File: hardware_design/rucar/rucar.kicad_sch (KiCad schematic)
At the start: 23 parts

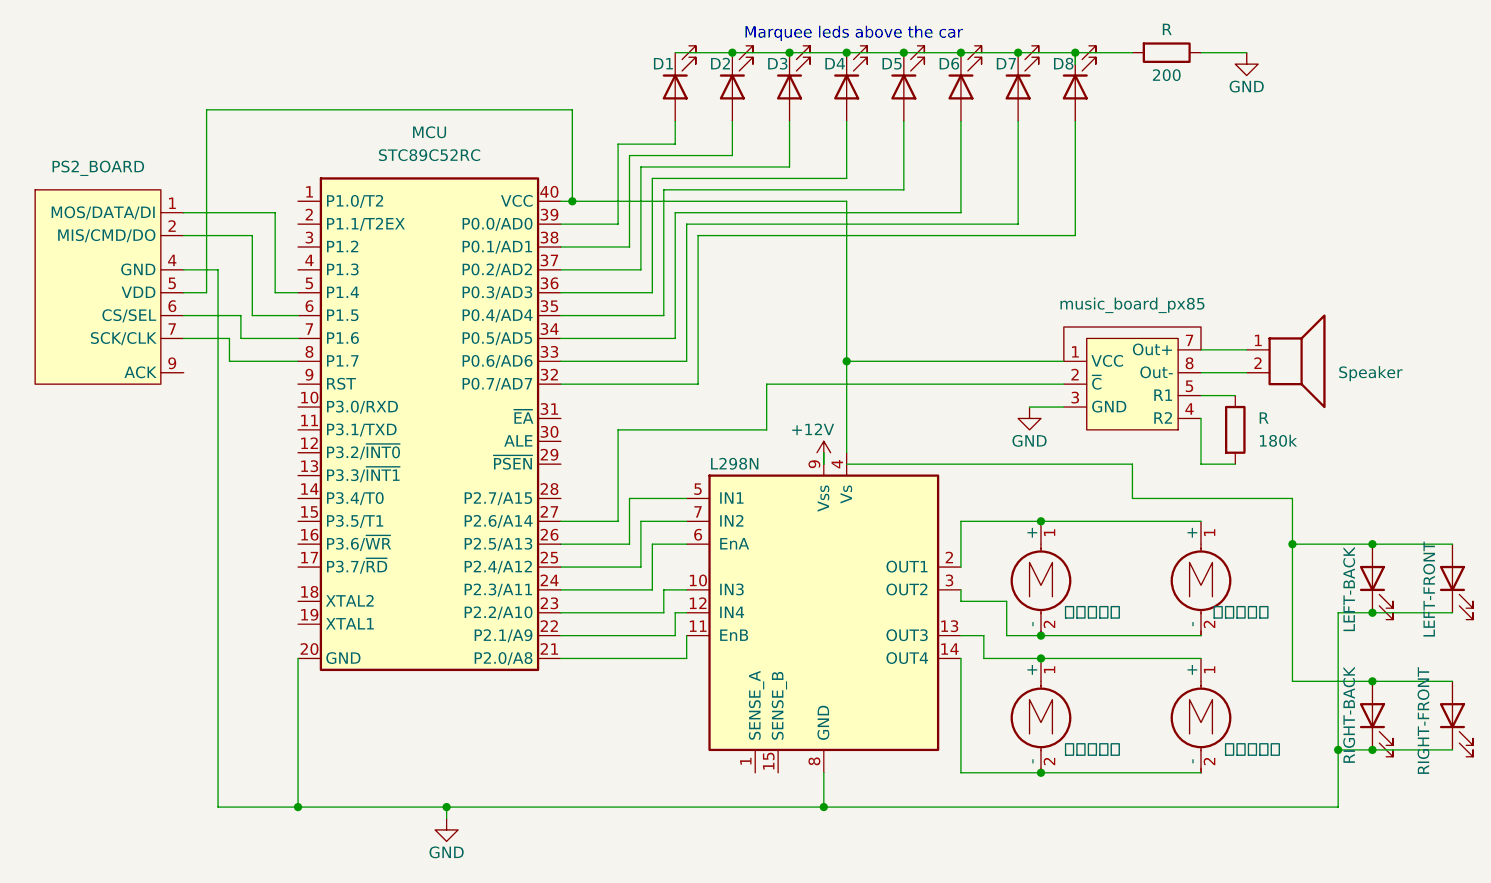
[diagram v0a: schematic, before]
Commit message: optimize
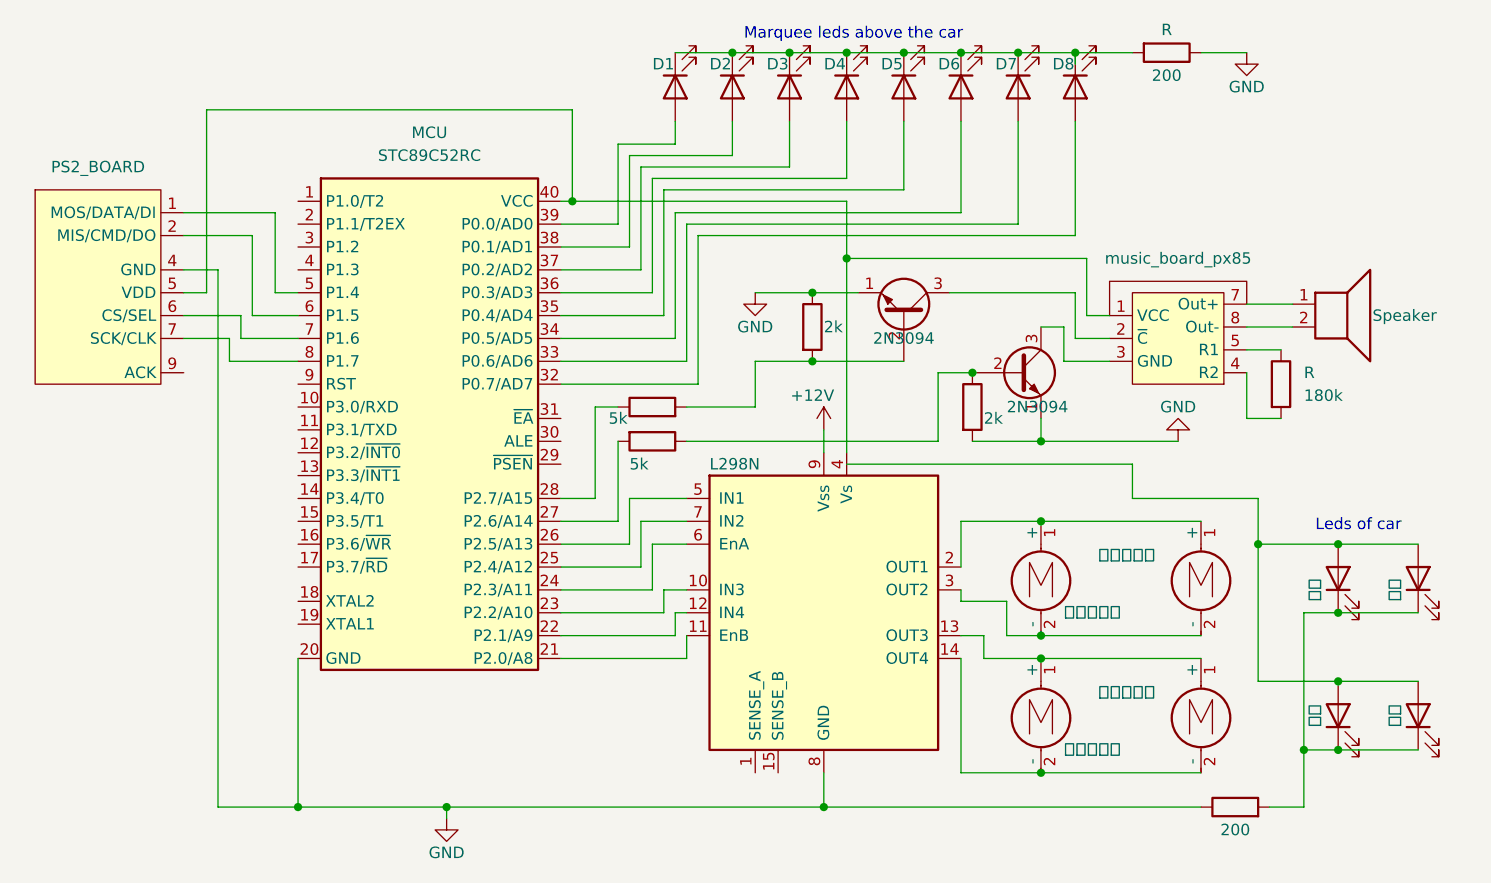
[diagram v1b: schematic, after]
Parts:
- added Q: 2N3094, Package_TO_SOT_THT:TO-92_Inline, symbol Transistor_BJT:2N3904
- added Q?: 2N3094, Package_TO_SOT_THT:TO-39-3, symbol Transistor_BJT:2N2219
- added R? (x2): 5k, symbol Device:R
- added R? (x2): 2k, symbol Device:R
- added R?: 200, symbol Device:R
- D: value RIGHT-FRONT -> 右前
- D: value LEFT-FRONT -> 左前
- D: value LEFT-BACK -> 左后
- D: value RIGHT-BACK -> 右后
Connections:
- net GND: now also Q.1 (E), Q?.1 (E), R?.1, R?.1, R?.2; no longer D.1 (K), D.1 (K), D.1 (K), D.1 (K), U?.3 (GND)
- net at MCU.27 (P2.6/A14): now also R?.2; no longer U?.2 (~{C})
- net at MCU.28 (P2.7/A15): now also R?.1
- new net: Q.2 (B), R?.1, R?.1
- new net: Q?.2 (B), R?.2, R?.2
- new net: Q?.3 (C), U?.2 (~{C})
- new net: Q.3 (C), U?.3 (GND)
- new net: D.1 (K), D.1 (K), D.1 (K), D.1 (K), R?.2
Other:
- note added: "Leds of car"
- moved on the sheet: R
